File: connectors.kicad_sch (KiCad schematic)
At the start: 23 parts, among them J12 USB_C, J13 2.5mm, J14 3.5mm, J3 GND spring, SW2 10k, U8 USBLC6-2SC6

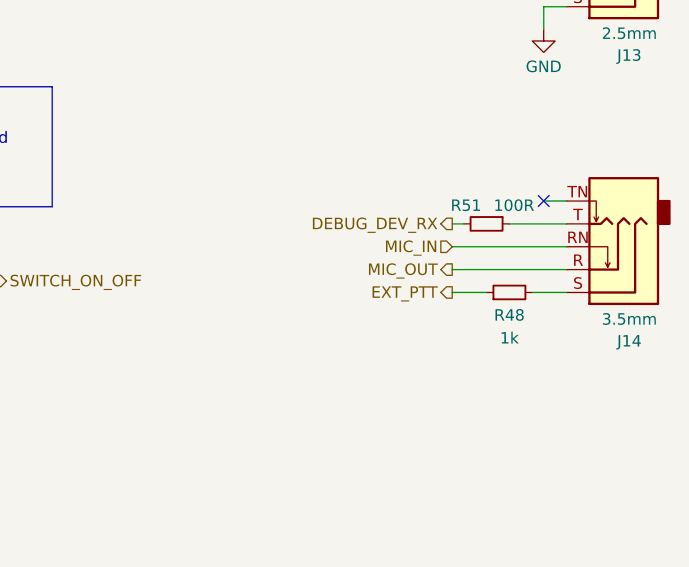
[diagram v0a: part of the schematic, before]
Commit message: Fixed wrong pinout on the 3.5 mm jack
RX signal is on the same pin as PTT on the Kenwood style connector.
This is used by many HT manufacturers, so for example Baofeng programming
cable can be used to connect to the debug UART of LinHT.

Fixes #31
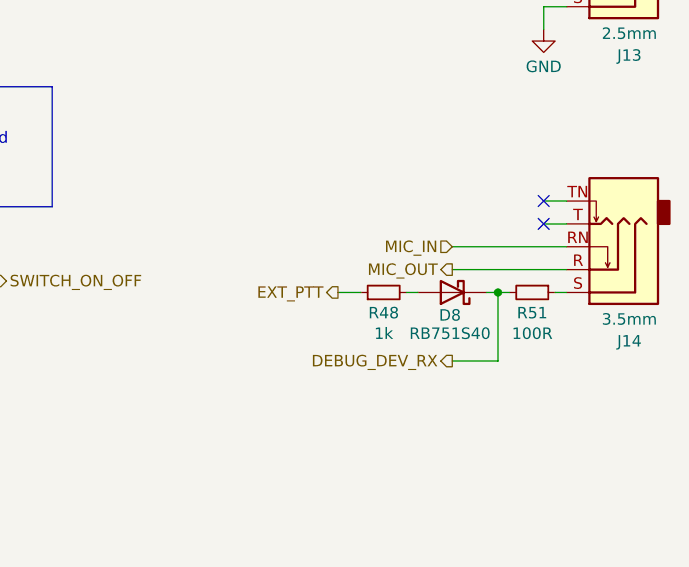
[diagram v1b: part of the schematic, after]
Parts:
- added D8: RB751S40, Diode_SMD:D_SOD-523, symbol Device:D_Schottky
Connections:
- net DEBUG_DEV_RX: now also D8.1 (K)
- net at R51.1: now also J14.S; no longer J14.T
- net at R48.2: now also D8.2 (A); no longer J14.S
- no-connect marks 4 -> 5
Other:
- moved on the sheet: R48, R51
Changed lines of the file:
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@@
+	)
+	(junction
+		(at 184.15 109.22)
+		(diameter 0)
+		(color 0 0 0 0)
 	)
 	(junction
@@
 		(at 54.61 163.83)
 	)
+	(no_connect
+		(at 189.23 101.6)
+	)
 	(wire
 		(pts
@@
 	(wire
 		(pts
-			(xy 187.96 109.22) (xy 191.77 109.22)
+			(xy 190.5 109.22) (xy 191.77 109.22)
 		)
 		(stroke
@@
 	(wire
 		(pts
+			(xy 184.15 109.22) (xy 185.42 109.22)
+		)
+		(stroke
+			(width 0)
+			(type default)
+		)
+	)
+	(wire
+		(pts
 			(xy 31.75 173.99) (xy 31.75 175.26)
 		)
@@
 	(wire
 		(pts
+			(xy 179.07 116.84) (xy 184.15 116.84)
+		)
+		(stroke
+			(width 0)
+			(type default)
+		)
+	)
+	(wire
+		(pts
 			(xy 189.23 99.06) (xy 191.77 99.06)
 		)
@@
 	(wire
 		(pts
-			(xy 185.42 101.6) (xy 191.77 101.6)
-		)
-		(stroke
-			(width 0)
-			(type default)
-		)
-	)
-	(wire
-		(pts
 			(xy 73.66 142.24) (xy 73.66 151.13)
 		)
@@
 	(wire
 		(pts
+			(xy 184.15 109.22) (xy 184.15 116.84)
+		)
+		(stroke
+			(width 0)
+			(type default)
+		)
+	)
+	(wire
+		(pts
 			(xy 54.61 140.97) (xy 57.15 140.97)
 		)
@@
 	(wire
 		(pts
+			(xy 189.23 101.6) (xy 191.77 101.6)
+		)
+		(stroke
+			(width 0)
+			(type default)
+		)
+	)
+	(wire
+		(pts
 			(xy 191.77 77.47) (xy 189.23 77.47)
 		)
@@
 	(wire
 		(pts
+			(xy 173.99 109.22) (xy 175.26 109.22)
+		)
+		(stroke
+			(width 0)
+			(type default)
+		)
+	)
+	(wire
+		(pts
 			(xy 54.61 151.13) (xy 57.15 151.13)
 		)
@@
 	(wire
 		(pts
-			(xy 179.07 109.22) (xy 182.88 109.22)
-		)
-		(stroke
-			(width 0)
-			(type default)
-		)
-	)
-	(wire
-		(pts
-			(xy 179.07 101.6) (xy 180.34 101.6)
+			(xy 182.88 109.22) (xy 184.15 109.22)
 		)
 		(stroke
@@
 			(width 0)
 			(type solid)
+		)
+	)
+	(wire
+		(pts
+			(xy 166.37 109.22) (xy 168.91 109.22)
+		)
+		(stroke
+			(width 0)
+			(type default)
 		)
 	)
@@
 	(hierarchical_label "EXT_PTT"
 		(shape output)
-		(at 179.07 109.22 180)
+		(at 166.37 109.22 180)
 		(effects
 			(font
@@
 	(hierarchical_label "DEBUG_DEV_RX"
 		(shape output)
-		(at 179.07 101.6 180)
+		(at 179.07 116.84 180)
 		(effects
 			(font
@@
 	)
 	(symbol
+		(lib_id "Device:D_Schottky")
+		(at 179.07 109.22 180)
+		(unit 1)
+		(exclude_from_sim no)
+		(in_bom yes)
+		(on_board yes)
+		(dnp no)
+		(property "Reference" "D8"
+			(at 178.816 111.76 0)
+			(effects
+				(font
+					(size 1.27 1.27)
+				)
+			)
+		)
+		(property "Value" "RB751S40"
+			(at 178.816 113.792 0)
+			(effects
+				(font
+					(size 1.27 1.27)
+				)
+			)
+		)
+		(property "Footprint" "Diode_SMD:D_SOD-523"
+			(at 179.07 109.22 0)
+			(effects
+				(font
+					(size 1.27 1.27)
+				)
+				(hide yes)
+			)
+		)
+		(property "Datasheet" "~"
+			(at 179.07 109.22 0)
+			(effects
+				(font
+					(size 1.27 1.27)
+				)
+				(hide yes)
+			)
+		)
+		(property "Description" "Schottky diode"
+			(at 179.07 109.22 0)
+			(effects
+				(font
+					(size 1.27 1.27)
+				)
+				(hide yes)
+			)
+		)
+		(property "Sim.Device" "D"
+			(at 179.07 109.22 0)
+			(effects
+				(font
+					(size 1.27 1.27)
+				)
+				(hide yes)
+			)
+		)
+		(property "Sim.Pins" "1=K 2=A"
+			(at 179.07 109.22 0)
+			(effects
+				(font
+					(size 1.27 1.27)
+				)
+				(hide yes)
+			)
+		)
+		(property "LCSC" "C5178963"
+			(at 179.07 109.22 0)
+			(effects
+				(font
+					(size 1.27 1.27)
+				)
+				(hide yes)
+			)
+		)
+		(property "MPN" "RB751S40T1G"
+			(at 179.07 109.22 0)
+			(effects
+				(font
+					(size 1.27 1.27)
+				)
+				(hide yes)
+			)
+		)
+		(property "PN" " 863-RB751S40T1G"
+			(at 179.07 109.22 0)
+			(effects
+				(font
+					(size 1.27 1.27)
+				)
+				(hide yes)
+			)
+		)
+		(pin "2"
+		)
+		(pin "1"
+		)
+		(instances
+			(project ""
+				(path "/73efc1fc-21f6-4aef-9f73-508fe18fa32e/5f168690-b6ac-4b3d-aad0-4e97277dc85d"
+					(reference "D8")
+					(unit 1)
+				)
+			)
+		)
+	)
+	(symbol
 		(lib_id "power:GND")
 		(at 72.39 153.67 270)
@@
 	(symbol
 		(lib_id "Device:R_Small")
-		(at 182.88 101.6 270)
+		(at 187.96 109.22 270)
 		(unit 1)
 		(exclude_from_sim no)
@@
 		(dnp no)
 		(property "Reference" "R51"
-			(at 180.594 99.568 90)
+			(at 187.96 111.506 90)
 			(effects
 				(font
@@
 		)
 		(property "Value" "100R"
-			(at 185.928 99.568 90)
+			(at 187.96 113.792 90)
 			(effects
 				(font
@@
 		)
 		(property "Footprint" "Resistor_SMD:R_0402_1005Metric"
-			(at 182.88 101.6 0)
+			(at 187.96 109.22 0)
 			(effects
 				(font
@@
 		)
 		(property "Datasheet" "~"
-			(at 182.88 101.6 0)
+			(at 187.96 109.22 0)
 			(effects
 				(font
@@
 		)
 		(property "Description" "Resistor, small symbol"
-			(at 182.88 101.6 0)
+			(at 187.96 109.22 0)
 			(effects
 				(font
@@
 		)
 		(property "PN" "0402WGF1000TCE"
-			(at 182.88 101.6 0)
+			(at 187.96 109.22 0)
 			(effects
 				(font
@@
 		)
 		(property "MPN" ""
-			(at 182.88 101.6 0)
+			(at 187.96 109.22 0)
 			(effects
 				(font
@@
 		)
 		(property "LCSC" "C25076"
-			(at 182.88 101.6 90)
+			(at 187.96 109.22 90)
 			(effects
 				(font
@@
 	(symbol
 		(lib_id "Device:R_Small")
-		(at 185.42 109.22 90)
+		(at 171.45 109.22 90)
 		(unit 1)
 		(exclude_from_sim no)
@@
 		(dnp no)
 		(property "Reference" "R48"
-			(at 185.42 111.76 90)
+			(at 171.45 111.506 90)
 			(effects
 				(font
@@
 		)
 		(property "Value" "1k"
-			(at 185.42 114.3 90)
+			(at 171.45 113.792 90)
 			(effects
 				(font
@@
 		)
 		(property "Footprint" "Resistor_SMD:R_0402_1005Metric"
-			(at 185.42 109.22 0)
+			(at 171.45 109.22 0)
 			(effects
 				(font
@@
 		)
 		(property "Datasheet" "~"
-			(at 185.42 109.22 0)
+			(at 171.45 109.22 0)
 			(effects
 				(font
@@
 		)
 		(property "Description" "Resistor, small symbol"
-			(at 185.42 109.22 0)
+			(at 171.45 109.22 0)
 			(effects
 				(font
@@
 		)
 		(property "PN" "0402WGF1001TCE"
-			(at 185.42 109.22 90)
+			(at 171.45 109.22 90)
 			(effects
 				(font
@@
 		)
 		(property "MPN" ""
-			(at 185.42 109.22 90)
+			(at 171.45 109.22 90)
 			(effects
 				(font
@@
 		)
 		(property "LCSC" "C11702"
-			(at 185.42 109.22 90)
-			(effects
-				(font
+			(at 171.45 109.22 90)
+			(effects
+				(font
